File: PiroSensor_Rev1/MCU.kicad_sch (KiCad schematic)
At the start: 9 parts, among them IC2 EFR32FG23L020F128GM40-C, J1 MY-18650-01, J2 MY-18650-01, Q1 AO3401A, SW1 SW_SPDT, SW2 SW_Push

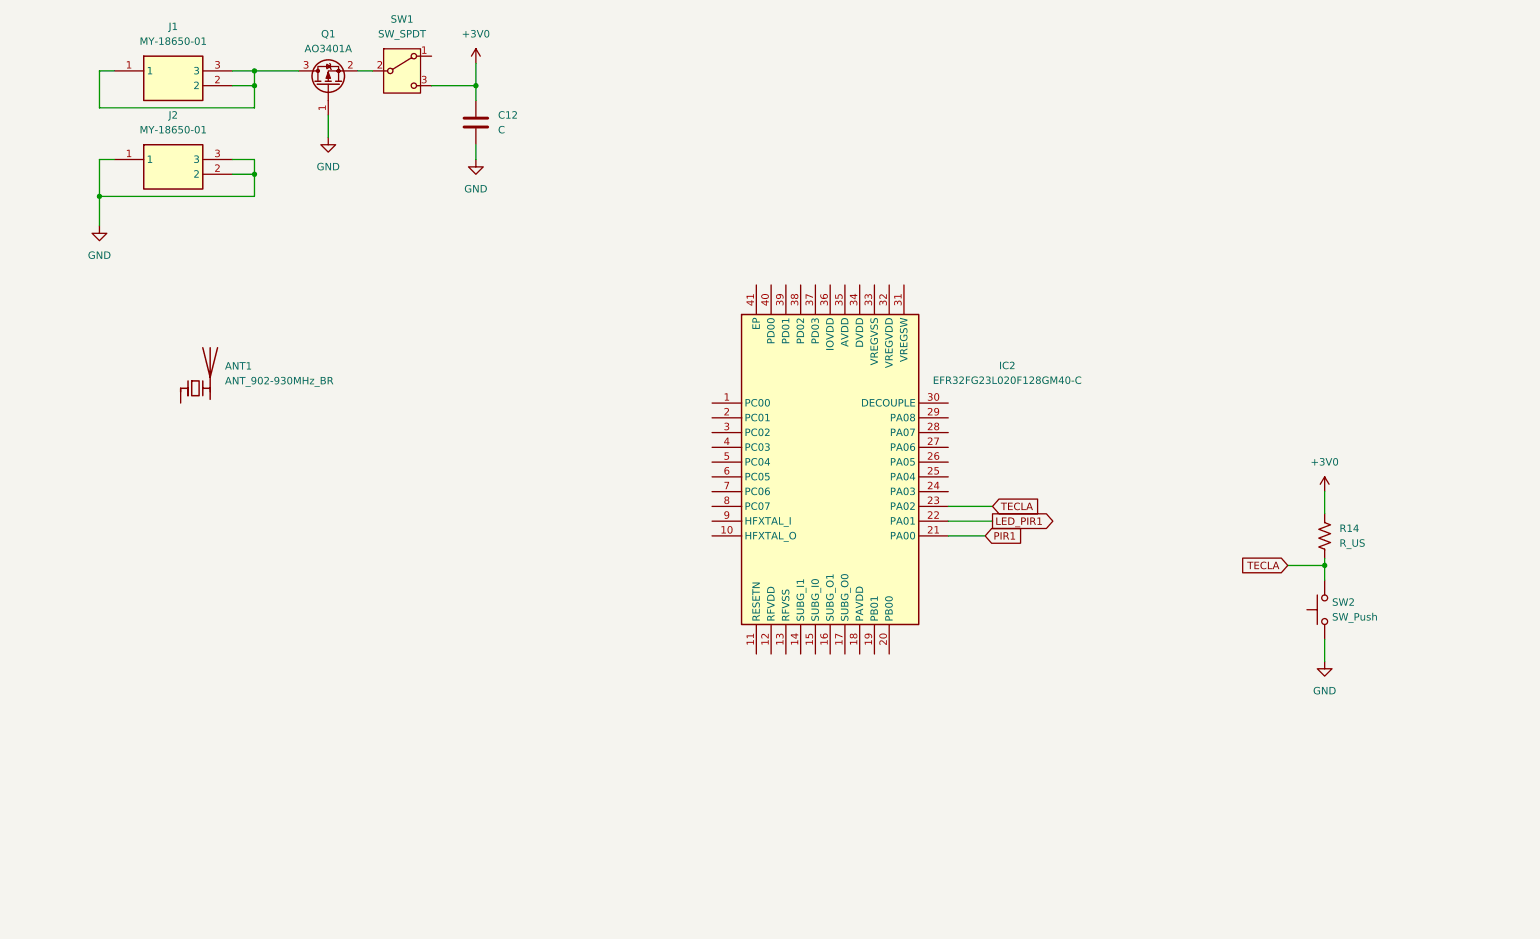
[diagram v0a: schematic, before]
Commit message: feat: atualização do projeto - 2026-06-05 15:12
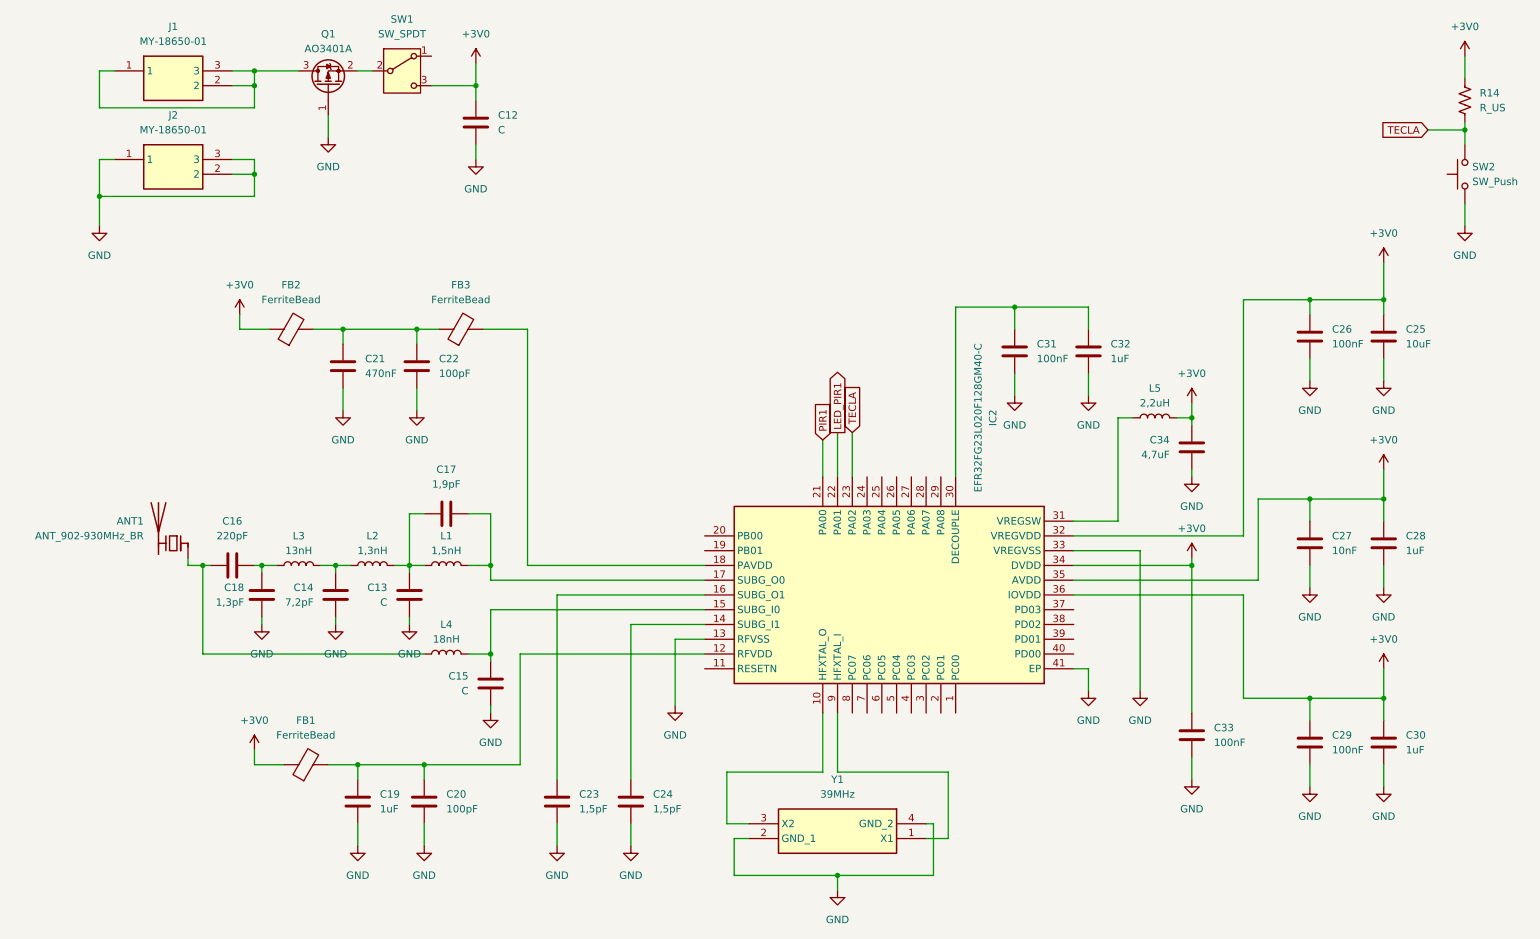
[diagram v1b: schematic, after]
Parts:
- added C13, C15: C, Capacitor_SMD:C_0603_1608Metric, symbol Device:C
- added C14: 7,2pF, Capacitor_SMD:C_0603_1608Metric, symbol Device:C
- added C16: 220pF, Capacitor_SMD:C_0603_1608Metric, symbol Device:C
- added C17: 1,9pF, Capacitor_SMD:C_0603_1608Metric, symbol Device:C
- added C18: 1,3pF, Capacitor_SMD:C_0603_1608Metric, symbol Device:C
- added C19, C28, C30, C32: 1uF, Capacitor_SMD:C_0603_1608Metric, symbol Device:C
- added C20, C22: 100pF, Capacitor_SMD:C_0603_1608Metric, symbol Device:C
- added C21: 470nF, Capacitor_SMD:C_0603_1608Metric, symbol Device:C
- added C23, C24: 1,5pF, Capacitor_SMD:C_0603_1608Metric, symbol Device:C
- added C25: 10uF, Capacitor_SMD:C_0603_1608Metric, symbol Device:C
- added C26, C29, C31, C33: 100nF, Capacitor_SMD:C_0603_1608Metric, symbol Device:C
- added C27: 10nF, Capacitor_SMD:C_0603_1608Metric, symbol Device:C
- added C34: 4,7uF, Capacitor_SMD:C_0603_1608Metric, symbol Device:C
- added FB1, FB2, FB3: FerriteBead, Inductor_SMD:L_0603_1608Metric, symbol Device:FerriteBead
- added L1: 1,5nH, Inductor_SMD:L_0603_1608Metric, symbol Device:L
- added L2: 1,3nH, Inductor_SMD:L_0603_1608Metric, symbol Device:L
- added L3: 13nH, Inductor_SMD:L_0603_1608Metric, symbol Device:L
- added L4: 18nH, Inductor_SMD:L_0603_1608Metric, symbol Device:L
- added L5: 2,2uH, Inductor_SMD:L_0603_1608Metric, symbol Device:L
- added Y1: 39MHz, ABM8AIG25000MHZ122ZT3, symbol SamacSys_Parts:ABM8AIG-25.000MHZ-12-2Z-T3
- SW2: footprint Button_Switch_SMD:SW_Push_1P1T_NO_CK_KSC6xxG -> Button_Switch_SMD:SW_Push_1P1T_NO_E-Switch_TL3301NxxxxxG
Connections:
- net +3V0: now also IC2.32 (VREGVDD), IC2.34 (DVDD), IC2.35 (AVDD), IC2.36 (IOVDD), C25.1, C26.1, C27.1, C28.1, C29.1, C30.1, C33.1, C34.1, FB1.1, FB2.1, L5.1
- net GND: now also IC2.13 (RFVSS), IC2.33 (VREGVSS), IC2.41 (EP), C13.2, C14.2, C15.2, C18.2, C19.2, C20.2, C21.2, C22.2, C23.2, C24.2, C25.2, C26.2, C27.2, C28.2, C29.2, C30.2, C31.2, C32.2, C33.2, C34.2, Y1.2 (GND_1), Y1.4 (GND_2)
- net at IC2.10 (HFXTAL_O): now also Y1.3 (X2)
- net at IC2.12 (RFVDD): now also C19.1, C20.1, FB1.2
- net at IC2.14 (SUBG_I1): now also C24.1
- net at IC2.15 (SUBG_I0): now also C15.1, L4.1
- net at IC2.16 (SUBG_O1): now also C23.1
- net at IC2.17 (SUBG_O0): now also C17.1, L1.1
- net at IC2.18 (PAVDD): now also FB3.2
- net at IC2.30 (DECOUPLE): now also C31.1, C32.1
- net at IC2.31 (VREGSW): now also L5.2
- net at IC2.9 (HFXTAL_I): now also Y1.1 (X1)
- net at ANT1.1 (FEED): now also C16.2, L4.2
- new net: C16.1, C18.1, L3.2
- new net: C13.1, C17.2, L1.2, L2.1
- new net: C21.1, C22.1, FB2.2, FB3.1
- new net: C14.1, L2.2, L3.1
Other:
- moved on the sheet: ANT1, IC2, R14
